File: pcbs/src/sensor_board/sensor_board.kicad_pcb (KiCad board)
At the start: 2 copper layers, 64 x 61 mm, 41 parts, among them J1 NPPN032AFCN-RCCONN3X2_NPPN032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, J2 NPPN032AFCN-RCCONN3X2_NPPN032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, U1 AP22818AKBWT, U2 AP22818AKBWT, U3 AP22818AKBWT, U4 AP22818AKBWT, U5 SN74AHCT1G125DBVR

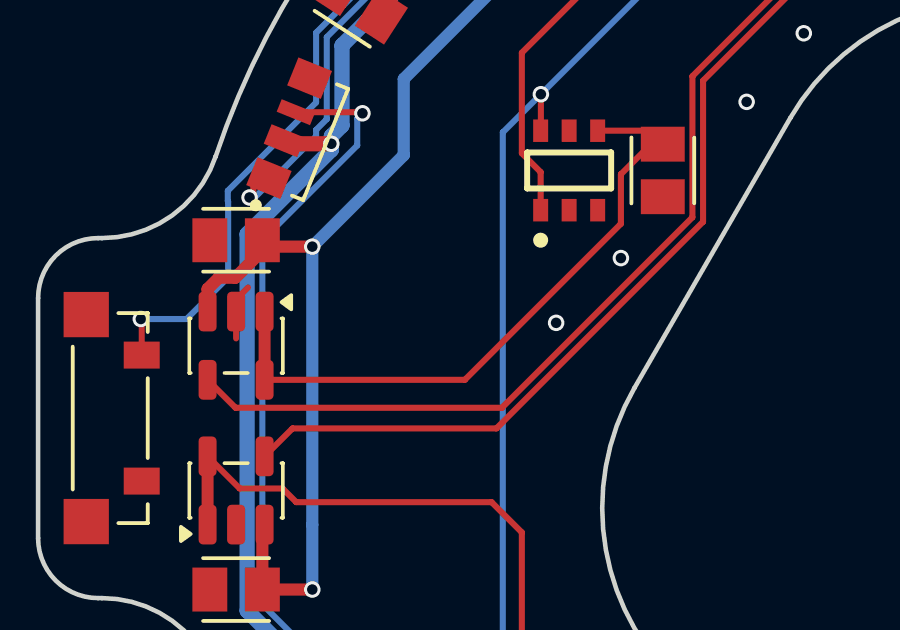
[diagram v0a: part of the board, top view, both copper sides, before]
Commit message: added gerbers
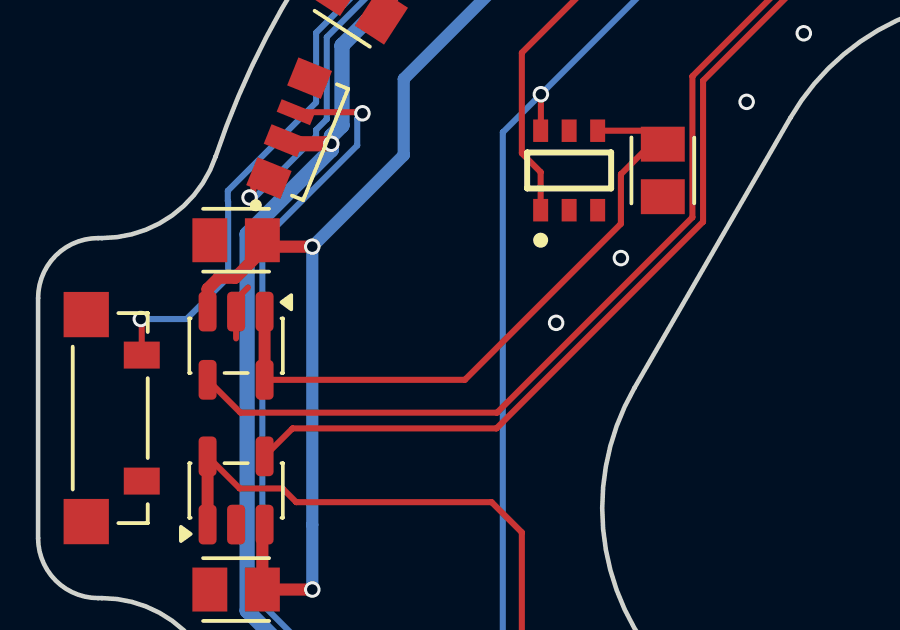
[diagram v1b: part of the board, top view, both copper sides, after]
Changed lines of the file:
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@@
 			(plot_on_all_layers_selection 0x00000000_00000000_00000000_00000000)
 			(disableapertmacros no)
-			(usegerberextensions no)
+			(usegerberextensions yes)
 			(usegerberattributes yes)
 			(usegerberadvancedattributes yes)
-			(creategerberjobfile yes)
+			(creategerberjobfile no)
 			(dashed_line_dash_ratio 12.000000)
 			(dashed_line_gap_ratio 3.000000)
@@
 			(outputformat 1)
 			(mirror no)
-			(drillshape 1)
+			(drillshape 0)
 			(scaleselection 1)
-			(outputdirectory "")
+			(outputdirectory "gerbers/")
 		)
 	)
@@
 	)
 	(segment
-		(start 138.31175 101.311513)
-		(end 131.963663 107.6596)
+		(start 146.925 91.775)
+		(end 146.925 92.525)
 		(width 0.2032)
 		(layer "F.Cu")
@@
 	)
 	(segment
-		(start 146.925 91.775)
-		(end 146.925 92.525)
+		(start 146.9201 92.5299)
+		(end 146.9201 93.0746)
 		(width 0.2032)
 		(layer "F.Cu")
@@
 	)
 	(segment
-		(start 131.963663 107.6596)
-		(end 123.082601 107.6596)
+		(start 123.246001 107.823)
+		(end 122.151101 106.7281)
 		(width 0.2032)
 		(layer "F.Cu")
@@
 	)
 	(segment
-		(start 141.6228 93.297)
-		(end 138.31175 96.60805)
+		(start 146.925 91)
+		(end 146.925 91.775)
 		(width 0.2032)
 		(layer "F.Cu")
@@
 	)
 	(segment
-		(start 123.082601 107.6596)
-		(end 122.151101 106.7281)
+		(start 131.800263 107.823)
+		(end 123.246001 107.823)
 		(width 0.2032)
 		(layer "F.Cu")
@@
 	)
 	(segment
-		(start 146.925 91)
-		(end 146.925 91.775)
+		(start 138.31175 96.60805)
+		(end 138.31175 101.311513)
 		(width 0.2032)
 		(layer "F.Cu")
@@
 	)
 	(segment
-		(start 138.31175 96.60805)
-		(end 138.31175 101.311513)
+		(start 146.6977 93.297)
+		(end 141.6228 93.297)
 		(width 0.2032)
 		(layer "F.Cu")
@@
 	)
 	(segment
-		(start 146.6977 93.297)
-		(end 141.6228 93.297)
+		(start 141.6228 93.297)
+		(end 138.31175 96.60805)
 		(width 0.2032)
 		(layer "F.Cu")
@@
 	)
 	(segment
-		(start 146.9201 92.5299)
-		(end 146.9201 93.0746)
+		(start 138.31175 101.311513)
+		(end 131.800263 107.823)
 		(width 0.2032)
 		(layer "F.Cu")
